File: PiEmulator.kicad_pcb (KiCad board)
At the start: 2 copper layers, 19 parts, among them J1 Conn_01x01, J2 Conn_01x01, J3 USB_C_Receptacle_USB2.0, U1 ADA3708, U3 BQ24090DGQ

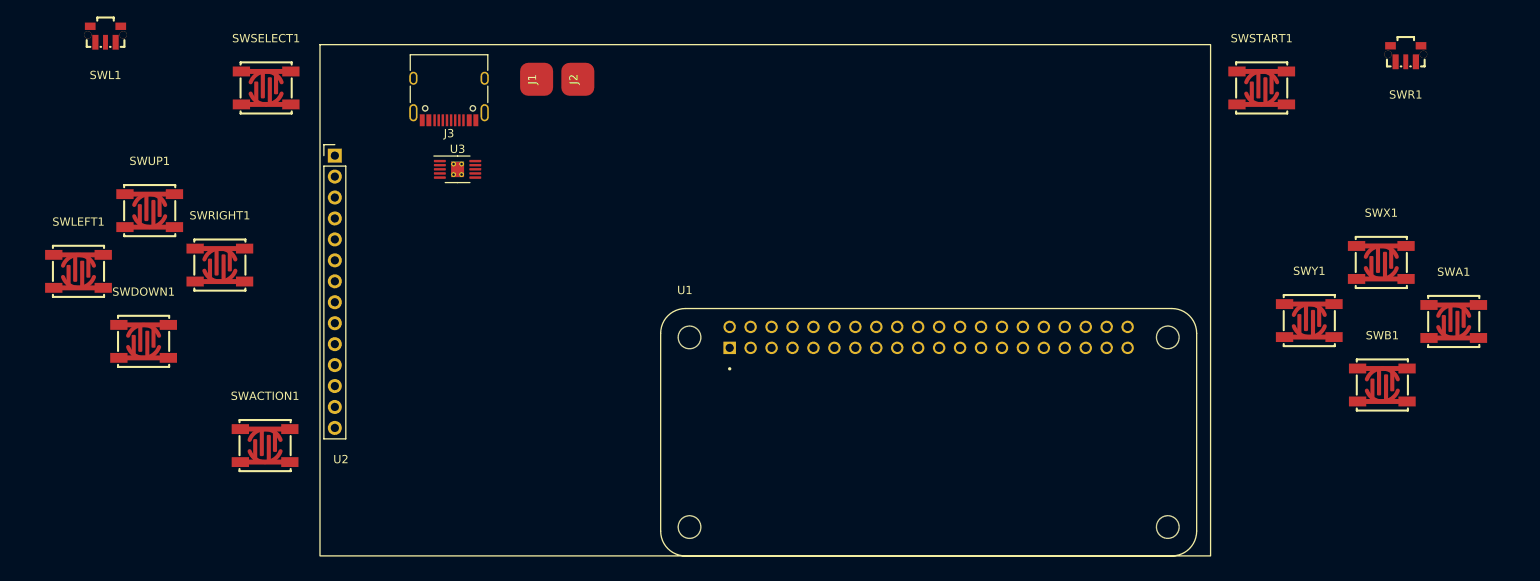
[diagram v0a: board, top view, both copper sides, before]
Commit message: routed
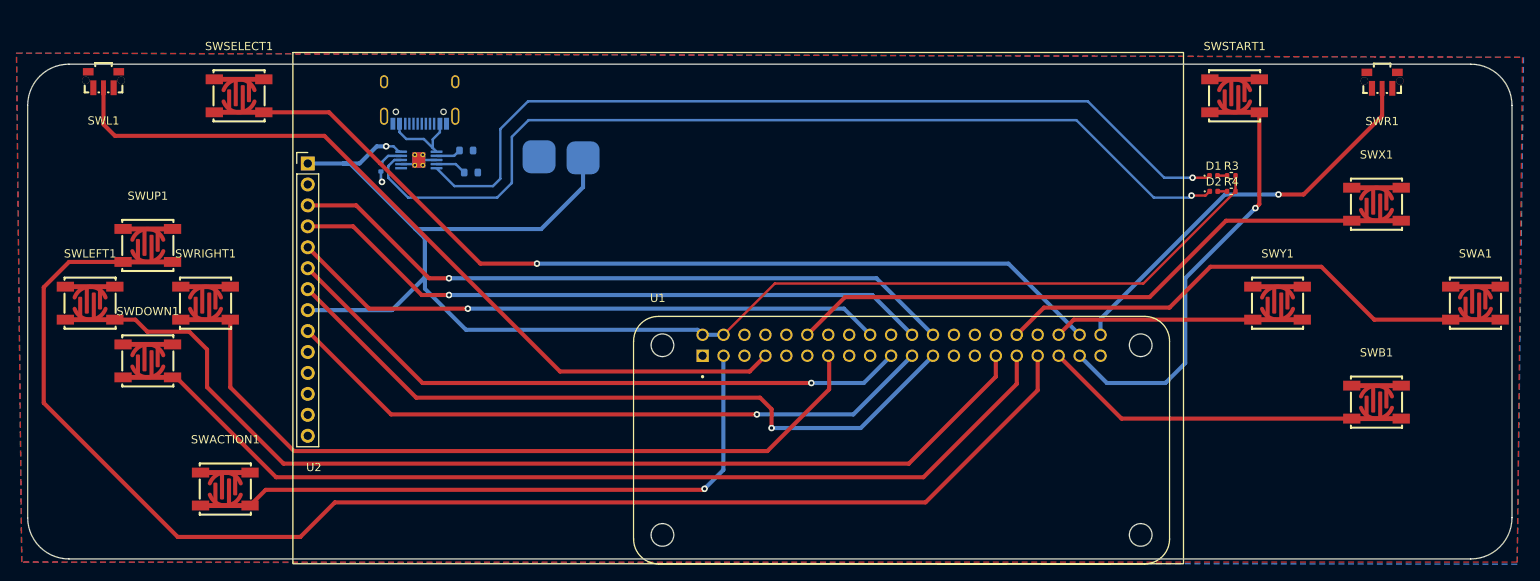
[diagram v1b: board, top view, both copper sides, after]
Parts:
- added D1: BLUE, LED_SMD:LED_0402_1005Metric, F.Cu at (181.9, 73.5)
- added D2: RED, LED_SMD:LED_0402_1005Metric, F.Cu at (181.9, 75.4)
- added R1: 540, Resistor_SMD:R_0603_1608Metric, B.Cu at (91.2, 70.5)
- added R2: 2K, Resistor_SMD:R_0603_1608Metric, B.Cu at (91.8, 73.2)
- added R3: 1K5, Resistor_SMD:R_0402_1005Metric, F.Cu at (184.0, 73.5)
- added R4: 1K5, Resistor_SMD:R_0402_1005Metric, F.Cu at (184.0, 75.4)
- added R5: 10K, Resistor_SMD:R_0402_1005Metric, B.Cu at (80.9, 72.5)
- J1, J2, J3, U3: moved to B.Cu
- moved J1 11.1 mm to (105.4, 71.4)
- moved J2 10.5 mm to (100.1, 71.2)
- moved SWACTION1 7.15 mm to (62.0, 111.5)
- moved SWX1 7.09 mm to (201.6, 77.0)
- moved SWL1 5.52 mm to (47.3, 61.9)
- moved SWRIGHT1 4.94 mm to (59.6, 89.0)
- moved U3 4.83 mm to (85.5, 71.6), turned to 180 degrees
- moved SWY1 4.39 mm to (189.6, 89.0)
- moved SWR1 4.31 mm to (202.3, 62.0)
- moved SWUP1 4.23 mm to (52.6, 82.0)
- moved SWLEFT1 4.11 mm to (45.6, 89.0)
- moved J3 3.58 mm to (85.6, 63.2), turned to 0 degrees
- moved SWA1 3.44 mm to (213.6, 89.0)
- moved SWSELECT1 3.42 mm to (63.7, 63.9)
- moved U1 3.42 mm to (144.0, 105.6)
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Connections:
- J1 pad 1: Net-(J1-Pin_1) -> +BATT
- U1 pad 12: /A -> /X
- U1 pad 13: unconnected-(U1-GPIO27_GEN2-Pad13) -> /Right
- U1 pad 14: unconnected-(U1-GND_4-Pad14) -> GND
- U1 pad 2: unconnected-(U1-5V_1-Pad2) -> +BATT
- U1 pad 20: unconnected-(U1-GND_5-Pad20) -> GND
- U1 pad 25: unconnected-(U1-GND_2-Pad25) -> GND
- U1 pad 29: /Right -> /Left
- U1 pad 3: /RB -> /Action
- U1 pad 30: /B -> GND
- U1 pad 31: /Left -> /Down
- U1 pad 32: /X -> /A
- U1 pad 33: /Down -> /Up
- U1 pad 34: unconnected-(U1-GND_7-Pad34) -> GND
- U1 pad 35: /Up -> /B
- U1 pad 39: unconnected-(U1-GND_3-Pad39) -> GND
- U1 pad 4: +5V -> +BATT
- U1 pad 40: /Action -> /RB
- U1 pad 9: unconnected-(U1-GND_1-Pad9) -> GND
- U2 pad 1: +5V -> +BATT
- U2 pad 8: +5V -> +BATT
- U3 pad 10: Net-(J1-Pin_1) -> +BATT
- U3 pad 7: unconnected-(U3-ISET2-Pad7) -> GND
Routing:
- net +BATT: track 0.00 -> 188.5 mm, vias 0 -> 1
- net /Up: track 0.00 -> 163.7 mm
- net /Left: track 0.00 -> 123.7 mm
- net /Down: track 0.00 -> 115.5 mm
- net Net-(D2-K): track 0.00 -> 115.3 mm, vias 0 -> 1
- net /Select: track 0.00 -> 110.1 mm, vias 0 -> 1
- net Net-(D1-K): track 0.00 -> 106.4 mm, vias 0 -> 1
- net /LB: track 0.00 -> 97.9 mm
- net /Right: track 0.00 -> 91.3 mm
- net /CLK: track 0.00 -> 87.8 mm, vias 0 -> 1
- net /CS: track 0.00 -> 82.3 mm, vias 0 -> 1
- net /MISO: track 0.00 -> 80.4 mm, vias 0 -> 1
- net /RESET: track 0.00 -> 78.7 mm, vias 0 -> 1
- net /MOSI: track 0.00 -> 77.9 mm, vias 0 -> 1
- net /Action: track 0.00 -> 73.0 mm, vias 0 -> 1
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- added copper zone on B.Cu, net GND
- added copper zone on F.Cu, net GND
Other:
- board outline added: 180 x 60 mm
